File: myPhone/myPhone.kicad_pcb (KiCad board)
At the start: 2 copper layers, 135 x 70 mm, 211 parts, among them J1 USB_OTG, J2 BATT, J201 ESP32.UART, J202 Modem, J203 SIM_Card, J204 Motor, J205 Micro_SD_Card, J206 Camera, J207 GPS, J3 RV.Debug, J301 iMX8, J4 SJ-3571N, J5 Display, J6 Touch, Q1 MMBT3906, SW1 RESET, SW2 WAKE, SW201 BOOT, U1 BQ25895, U10 74HC595, U11 ICS-43434, U12 MAX98357A, U13 FT813Q, U14 FAN5333BSX, U2 TPS62293, U201 ESP32-WROOM, U202 SN74CBTLV3125, U203 TXB0104RGY, U204 TXB0104RGY, U205 DRV2605L, U206 SN74CBTLV3126, U207 TPS22917, U208 SN74LVC2G66, U209 TPS22917, U3 TPS630250, U4 SN74LVC2G07, U5 E310-G000, U6 IS25LP128-JBLE, U7 74HC00, U8 74HC00, U9 74HC595, X1 SiT1533, Y1 16MHz, Y2 12MHz

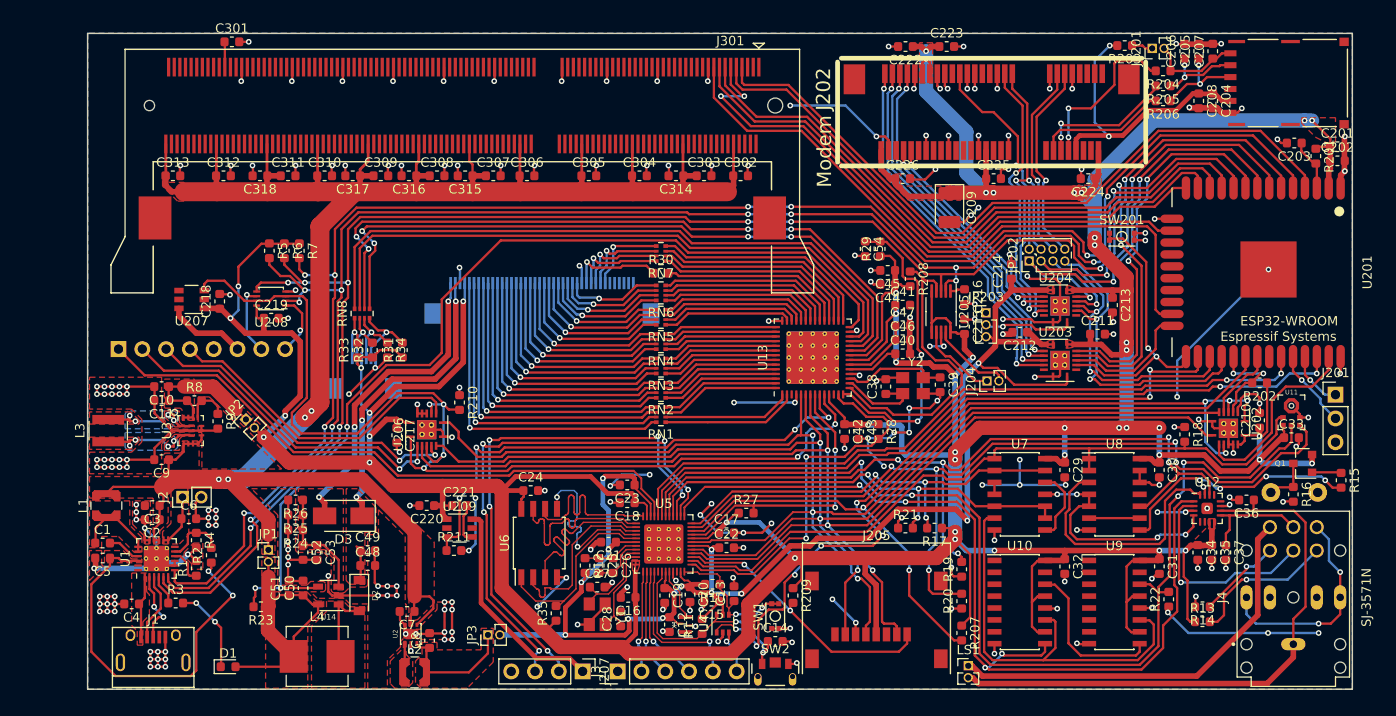
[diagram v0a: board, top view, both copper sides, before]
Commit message: REV1 board
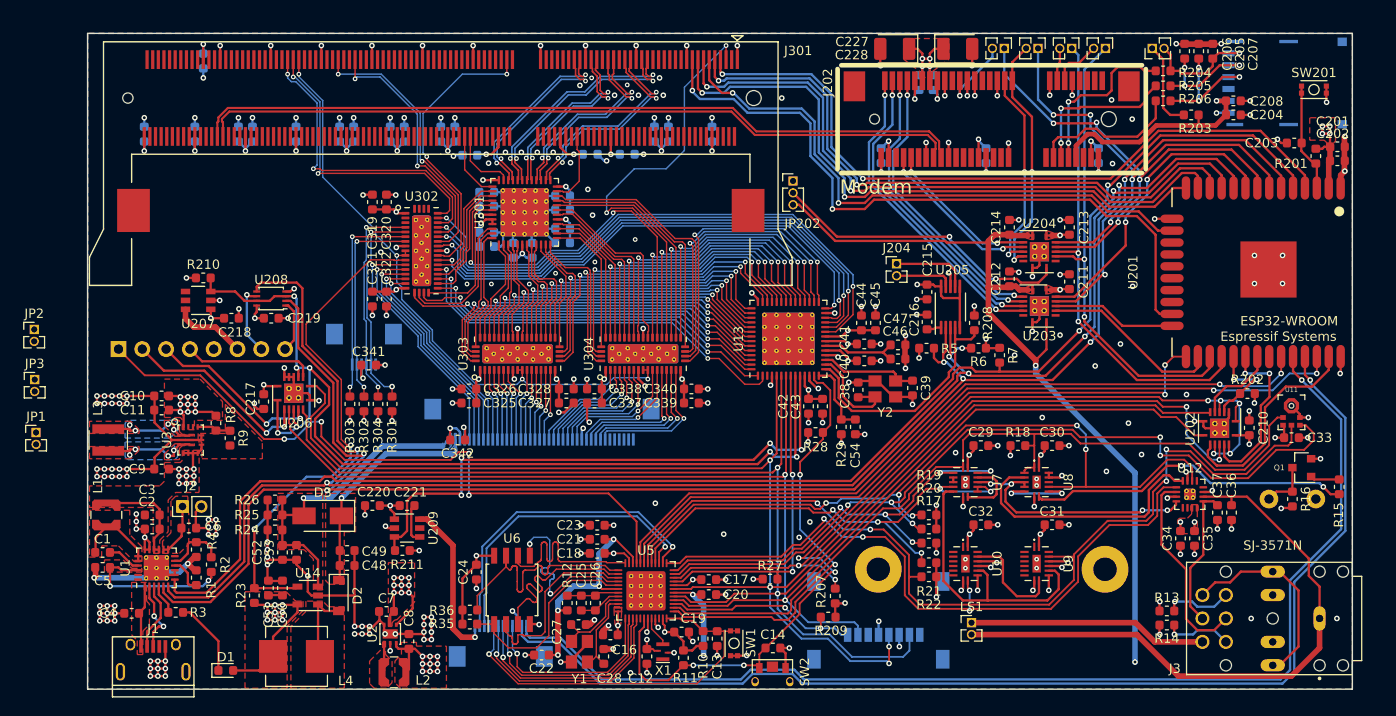
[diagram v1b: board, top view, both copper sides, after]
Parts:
- removed C15: 0.1uF, Capacitor_SMD:C_0603_1608Metric
- removed C209: 470uF, Capacitor_Tantalum_SMD:CP_EIA-3528-21_Kemet-B
- removed J201: ESP32.UART, Connector_PinHeader_2.54mm:PinHeader_1x03_P2.54mm_Vertical
- removed J207: GPS, Connector_PinHeader_2.54mm:PinHeader_1x04_P2.54mm_Vertical
- removed J4: SJ-3571N, footprints:CUI_SJ-3571N
- removed J5: Display, footprints:Hirose_FH12-40S-0.5SH_1x40-1MP_P0.50mm_Horizontal_Bottom
- removed J6: Touch, footprints:Hirose_FH12-6S-0.5SH_1x06-1MP_P0.50mm_Horizontal_Bottom
- removed the JP202 at (197.7, 96.1)
- removed R30: 33R, Resistor_SMD:R_0603_1608Metric
- removed RN1, RN2, RN3, RN4, RN5, RN6, RN7, RN8: 33R, footprints:R_Array_Convex_4x0402
- removed U4: SN74LVC2G07, Package_TO_SOT_SMD:SOT-363_SC-70-6
- added C227: 470uF, Capacitor_Tantalum_SMD:CP_EIA-3528-21_Kemet-B, F.Cu at (190.1, 73.5)
- added C228: 470uF, Capacitor_Tantalum_SMD:CP_EIA-3528-21_Kemet-B, F.Cu at (183.3, 73.5)
- added C319: 1uF, Capacitor_SMD:C_0603_1608Metric, F.Cu at (127.6, 89.8)
- added C320: 0.1uF, Capacitor_SMD:C_0603_1608Metric, F.Cu at (129.1, 89.8)
- added C321: 1uF, Capacitor_SMD:C_0603_1608Metric, F.Cu at (127.6, 100.2)
- added C322: 0.1uF, Capacitor_SMD:C_0603_1608Metric, F.Cu at (129.1, 100.2)
- added C323: 0.1uF, Capacitor_SMD:C_0603_1608Metric, B.Cu at (147.9, 90.7)
- added C324: 0.01uF, Capacitor_SMD:C_0603_1608Metric, B.Cu at (147.9, 89.2)
- added C325: 1uF, Capacitor_SMD:C_0603_1608Metric, F.Cu at (137.9, 111.2)
- added C326: 0.1uF, Capacitor_SMD:C_0603_1608Metric, F.Cu at (137.9, 109.8)
- added C327: 1uF, Capacitor_SMD:C_0603_1608Metric, F.Cu at (148.3, 111.2)
- added C328: 0.1uF, Capacitor_SMD:C_0603_1608Metric, F.Cu at (148.3, 109.8)
- added C329: 0.1uF, Capacitor_SMD:C_0603_1608Metric, B.Cu at (139.8, 94.5)
- added C330: 0.01uF, Capacitor_SMD:C_0603_1608Metric, B.Cu at (139.8, 93.0)
- added C331: 0.1uF, Capacitor_SMD:C_0603_1608Metric, B.Cu at (142.7, 95.0)
- added C332: 0.01uF, Capacitor_SMD:C_0603_1608Metric, B.Cu at (144.7, 95.0)
- added C333: 0.1uF, Capacitor_SMD:C_0603_1608Metric, B.Cu at (147.9, 94.2)
- added C334: 0.01uF, Capacitor_SMD:C_0603_1608Metric, B.Cu at (147.9, 92.7)
- added C335: 0.1uF, Capacitor_SMD:C_0603_1608Metric, B.Cu at (139.8, 88.8)
- added C336: 0.01uF, Capacitor_SMD:C_0603_1608Metric, B.Cu at (139.8, 90.2)
- added C337: 1uF, Capacitor_SMD:C_0603_1608Metric, F.Cu at (151.3, 111.2)
- added C338: 0.1uF, Capacitor_SMD:C_0603_1608Metric, F.Cu at (151.3, 109.8)
- added C339: 1uF, Capacitor_SMD:C_0603_1608Metric, F.Cu at (161.7, 111.2)
- added C340: 0.1uF, Capacitor_SMD:C_0603_1608Metric, F.Cu at (161.7, 109.8)
- added C341: 0.1uF, Capacitor_SMD:C_0603_1608Metric, F.Cu at (127.2, 107.2)
- added C342: 0.1uF, Capacitor_SMD:C_0603_1608Metric, F.Cu at (136.7, 115.2)
- added J302: Touch, Connector_FFC-FPC:Hirose_FH12-6S-0.5SH_1x06-1MP_P0.50mm_Horizontal, B.Cu at (126.7, 105.3)
- added J303: Display, Connector_FFC-FPC:Hirose_FH12-40S-0.5SH_1x40-1MP_P0.50mm_Horizontal, B.Cu at (145.7, 113.3)
- added J304: Prog, Connector_FFC-FPC:Hirose_FH12-12S-0.5SH_1x12-1MP_P0.50mm_Horizontal, B.Cu at (141.3, 136.9)
- added JP203: Q.DTR, Connector_PinHeader_1.27mm:PinHeader_1x02_P1.27mm_Vertical, F.Cu at (195.1, 73.4)
- added JP204: Q.RI, Connector_PinHeader_1.27mm:PinHeader_1x02_P1.27mm_Vertical, F.Cu at (198.7, 73.4)
- added JP205: Q.TXD, Connector_PinHeader_1.27mm:PinHeader_1x02_P1.27mm_Vertical, F.Cu at (202.2, 73.4)
- added JP206: Q.RXD, Connector_PinHeader_1.27mm:PinHeader_1x02_P1.27mm_Vertical, F.Cu at (205.8, 73.4)
- added R36: 100K, Resistor_SMD:R_0603_1608Metric, F.Cu at (138.0, 133.3)
- added U301: SN65LVDS822_SWAP, Package_DFN_QFN:QFN-48-1EP_7x7mm_P0.5mm_EP5.15x5.15mm_ThermalVias, F.Cu at (143.8, 90.9)
- added U302: TS3DDR3812, footprints:Texas_R-PWQFN-N42, F.Cu at (132.8, 95.0)
- added U303: TS3DDR3812, footprints:Texas_R-PWQFN-N42, F.Cu at (143.1, 106.0)
- added U304: TS3DDR3812, footprints:Texas_R-PWQFN-N42, F.Cu at (156.5, 106.0)
- C222, C223, C224, C225, C226, C301, C302, C303, C304, C305, C306, C307, C308, C309, C310, C311, C312, C313, C314, C315, C316, C317, C318, J203, J205: moved to B.Cu
- J3: value RV.Debug -> SJ-3571N; footprint Connector_PinHeader_2.54mm:PinHeader_1x06_P2.54mm_Vertical -> footprints:CUI_SJ-3571N
- R208: value 47K -> 100K
- U10, U9: footprint Package_SO:SOIC-16_3.9x9.9mm_P1.27mm -> footprints:74HC595BQ115
- U12: footprint Package_DFN_QFN:TQFN-16-1EP_3x3mm_P0.5mm_EP1.23x1.23mm -> footprints:TQFN-16-1EP_3x3mm_P0.5mm_EP1.23x1.23mm_ThermalVias
- U5: value E310-G000 -> E310-G002
- U7, U8: footprint Package_SO:SOIC-14_3.9x8.7mm_P1.27mm -> footprints:74HC00BQ115
- moved R7 75.6 mm to (194.6, 106.2)
- moved R6 74.8 mm to (192.3, 105.4), turned to 180 degrees
- moved R5 70.9 mm to (186.8, 105.4), turned to 0 degrees
- moved J3 70.1 mm to (223.7, 134.2), turned to 180 degrees
- moved JP3 55.5 mm to (91.5, 108.8), turned to 0 degrees
- moved R210 30.4 mm to (109.5, 97.9), turned to 0 degrees
- moved JP1 27.8 mm to (91.7, 114.4)
- moved SW201 25.8 mm to (228.1, 77.8)
- moved R22 25.7 mm to (187.0, 129.8), turned to 180 degrees
- moved JP202 25.0 mm to (172.5, 87.5)
- moved JP2 24.6 mm to (91.5, 103.4), turned to 0 degrees
- moved R29 19.4 mm to (177.7, 113.8)
- moved C54 19.0 mm to (179.2, 113.8)
- moved R18 17.8 mm to (196.5, 115.8), turned to 0 degrees
- moved J204 15.8 mm to (183.6, 96.4), turned to 0 degrees
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- renumbered C20 to C19, C22 to C20, C23 to C21, C19 to C22, C21 to C23, JP203 to JP202, R31 to R301, R32 to R302, R33 to R303, R34 to R304
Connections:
- net /DISP_LED_A renamed DISP_LED_A
- net /DISP_LED_K renamed DISP_LED_K
- net Net-(C25-Pad2) renamed /PLL_AVSS
- net Net-(C27-Pad1) renamed /XTAL_XI
- net Net-(C28-Pad1) renamed /XTAL_XO
- net Net-(R35-Pad2) renamed /QSPI_CS
- net Net-(U5-Pad1) renamed /QSPI_DQ_3
- net Net-(U5-Pad2) renamed /QSPI_DQ_2
- net Net-(U5-Pad20) renamed /PSD_LFALTCLK
- net Net-(U5-Pad3) renamed /QSPI_DQ_1
- net Net-(U5-Pad4) renamed /QSPI_DQ_0
- net Net-(U5-Pad48) renamed /QSPI_CLK
- C12 pad 1: +1V8 -> +3V3
- C13 pad 1: Net-(C13-Pad1) -> RESET
- C14 pad 1: Net-(C14-Pad1) -> WAKE
- C19 pad 1: +1V8 -> +3V3
- C23 pad 1: +1V8 -> +3V3
- C25 pad 1: Net-(C25-Pad1) -> /PLL_AVDD
- C26 pad 1: Net-(C25-Pad1) -> /PLL_AVDD
- J1 pad 4: (no net) -> Net-(J1-Pad4)
- J202 pad 1: (no net) -> Net-(J202-Pad1)
- J202 pad 16: (no net) -> Net-(J202-Pad16)
- J202 pad 20: (no net) -> Net-(J202-Pad20)
- J202 pad 22: (no net) -> Net-(J202-Pad22)
- J202 pad 23: (no net) -> Net-(J202-Pad23)
- J202 pad 25: (no net) -> Net-(J202-Pad25)
- J202 pad 28: (no net) -> Net-(J202-Pad28)
- J202 pad 3: (no net) -> Net-(J202-Pad3)
- J202 pad 30: (no net) -> Net-(J202-Pad30)
- J202 pad 32: (no net) -> Net-(J202-Pad32)
- J202 pad 33: (no net) -> Net-(J202-Pad33)
- J202 pad 36: (no net) -> iMX8_USB1_D_N
- J202 pad 38: (no net) -> iMX8_USB1_D_P
- J202 pad 42: (no net) -> Net-(J202-Pad42)
- J202 pad 48: (no net) -> Net-(J202-Pad48)
- J202 pad 5: (no net) -> Net-(J202-Pad5)
- J202 pad 6: (no net) -> Net-(J202-Pad6)
- J202 pad 7: (no net) -> Net-(J202-Pad7)
- J203 pad 6: (no net) -> Net-(J203-Pad6)
- J205 pad 3: (no net) -> Net-(J205-Pad3)
- J205 pad 8: (no net) -> Net-(J205-Pad8)
- J3 pad 1: GND -> /SPK_VO-
- J3 pad 2: JTAG_TCK -> Net-(J3-Pad2)
- J3 pad 3: JTAG_TDO -> Net-(J3-Pad2)
- J3 pad 4: JTAG_TMS -> Net-(J3-Pad4)
- J3 pad 5: JTAG_TDI -> /SPK_GAIN
- J3 pad 6: RESET -> Net-(J3-Pad6)
- J301 pad 100: (no net) -> Net-(J301-Pad100)
- J301 pad 101: (no net) -> Net-(J301-Pad101)
- J301 pad 102: (no net) -> Net-(J301-Pad102)
- J301 pad 103: (no net) -> Net-(J301-Pad103)
- J301 pad 104: (no net) -> Net-(J301-Pad104)
- J301 pad 106: (no net) -> Net-(J301-Pad106)
- J301 pad 107: (no net) -> Net-(J301-Pad107)
- J301 pad 108: (no net) -> Net-(J301-Pad108)
- J301 pad 109: (no net) -> Net-(J301-Pad109)
- J301 pad 110: (no net) -> Net-(J301-Pad110)
- J301 pad 111: (no net) -> Net-(J301-Pad111)
- J301 pad 112: (no net) -> Net-(J301-Pad112)
- J301 pad 113: (no net) -> Net-(J301-Pad113)
- J301 pad 115: (no net) -> Net-(J301-Pad115)
- J301 pad 116: (no net) -> Net-(J301-Pad116)
- J301 pad 117: (no net) -> Net-(J301-Pad117)
- J301 pad 118: (no net) -> Net-(J301-Pad118)
- J301 pad 119: (no net) -> Net-(J301-Pad119)
- J301 pad 12: (no net) -> Net-(J301-Pad12)
- J301 pad 120: (no net) -> Net-(J301-Pad120)
- J301 pad 121: (no net) -> Net-(J301-Pad121)
- J301 pad 122: (no net) -> Net-(J301-Pad122)
- J301 pad 124: (no net) -> Net-(J301-Pad124)
- J301 pad 125: (no net) -> Net-(J301-Pad125)
- J301 pad 126: (no net) -> Net-(J301-Pad126)
- J301 pad 127: (no net) -> Net-(J301-Pad127)
- J301 pad 128: (no net) -> Net-(J301-Pad128)
- J301 pad 129: (no net) -> iMX8_I2C1_SCL
- J301 pad 130: (no net) -> Net-(J301-Pad130)
- J301 pad 131: (no net) -> Net-(J301-Pad131)
- J301 pad 133: (no net) -> Net-(J301-Pad133)
- J301 pad 134: (no net) -> Net-(J301-Pad134)
- J301 pad 135: (no net) -> iMX8_I2C1_SDA
- J301 pad 136: (no net) -> Net-(J301-Pad136)
- J301 pad 137: (no net) -> Net-(J301-Pad137)
- J301 pad 138: (no net) -> Net-(J301-Pad138)
- J301 pad 139: (no net) -> Net-(J301-Pad139)
- J301 pad 14: (no net) -> Net-(J301-Pad14)
- J301 pad 140: (no net) -> Net-(J301-Pad140)
- J301 pad 142: (no net) -> Net-(J301-Pad142)
- J301 pad 143: (no net) -> Net-(J301-Pad143)
- J301 pad 144: (no net) -> Net-(J301-Pad144)
- J301 pad 145: (no net) -> Net-(J301-Pad145)
- J301 pad 146: (no net) -> Net-(J301-Pad146)
- J301 pad 147: (no net) -> Net-(J301-Pad147)
- J301 pad 148: (no net) -> Net-(J301-Pad148)
- J301 pad 149: (no net) -> iMX8_GPIO3_IO13
- J301 pad 151: (no net) -> iMX8_GPIO3_IO12
- J301 pad 152: (no net) -> Net-(J301-Pad152)
- J301 pad 153: (no net) -> iMX8_GPIO3_IO11
- J301 pad 154: (no net) -> Net-(J301-Pad154)
- J301 pad 155: (no net) -> Net-(J301-Pad155)
- J301 pad 156: (no net) -> Net-(J301-Pad156)
- J301 pad 157: (no net) -> Net-(J301-Pad157)
- J301 pad 158: (no net) -> Net-(J301-Pad158)
- J301 pad 16: (no net) -> Net-(J301-Pad16)
- J301 pad 160: (no net) -> Net-(J301-Pad160)
- J301 pad 161: (no net) -> Net-(J301-Pad161)
- J301 pad 162: (no net) -> Net-(J301-Pad162)
- J301 pad 163: (no net) -> Net-(J301-Pad163)
- J301 pad 164: (no net) -> Net-(J301-Pad164)
- J301 pad 165: (no net) -> Net-(J301-Pad165)
- J301 pad 166: (no net) -> Net-(J301-Pad166)
- J301 pad 167: (no net) -> Net-(J301-Pad167)
- J301 pad 169: (no net) -> Net-(J301-Pad169)
- J301 pad 170: (no net) -> Net-(J301-Pad170)
- J301 pad 171: (no net) -> Net-(J301-Pad171)
- J301 pad 172: (no net) -> Net-(J301-Pad172)
- J301 pad 173: (no net) -> Net-(J301-Pad173)
- J301 pad 174: (no net) -> Net-(J301-Pad174)
- J301 pad 175: (no net) -> Net-(J301-Pad175)
- J301 pad 176: (no net) -> iMX8_USB1_D_P
- J301 pad 178: (no net) -> iMX8_USB1_D_N
- J301 pad 179: (no net) -> Net-(J301-Pad179)
- J301 pad 18: (no net) -> Net-(J301-Pad18)
- J301 pad 180: (no net) -> Net-(J301-Pad180)
- J301 pad 181: (no net) -> Net-(J301-Pad181)
- J301 pad 182: (no net) -> Net-(J301-Pad182)
- J301 pad 184: (no net) -> Net-(J301-Pad184)
- J301 pad 185: (no net) -> Net-(J301-Pad185)
- J301 pad 187: (no net) -> Net-(J301-Pad187)
- J301 pad 188: (no net) -> Net-(J301-Pad188)
- J301 pad 189: (no net) -> Net-(J301-Pad189)
- J301 pad 190: (no net) -> Net-(J301-Pad190)
- J301 pad 191: (no net) -> Net-(J301-Pad191)
- J301 pad 192: (no net) -> Net-(J301-Pad192)
- J301 pad 193: (no net) -> Net-(J301-Pad193)
- J301 pad 194: (no net) -> Net-(J301-Pad194)
- J301 pad 195: (no net) -> Net-(J301-Pad195)
- J301 pad 196: (no net) -> Net-(J301-Pad196)
- J301 pad 197: (no net) -> Net-(J301-Pad197)
- J301 pad 198: (no net) -> Net-(J301-Pad198)
- J301 pad 199: (no net) -> Net-(J301-Pad199)
- J301 pad 2: (no net) -> Net-(J301-Pad2)
- J301 pad 20: (no net) -> Net-(J301-Pad20)
- J301 pad 200: (no net) -> Net-(J301-Pad200)
- J301 pad 201: (no net) -> Net-(J301-Pad201)
- J301 pad 202: (no net) -> Net-(J301-Pad202)
- J301 pad 203: (no net) -> Net-(J301-Pad203)
- J301 pad 21: (no net) -> Net-(J301-Pad21)
- J301 pad 22: (no net) -> Net-(J301-Pad22)
- J301 pad 23: (no net) -> Net-(J301-Pad23)
- J301 pad 24: (no net) -> Net-(J301-Pad24)
- J301 pad 25: (no net) -> Net-(J301-Pad25)
- J301 pad 26: (no net) -> Net-(J301-Pad26)
- J301 pad 27: (no net) -> Net-(J301-Pad27)
- J301 pad 29: (no net) -> Net-(J301-Pad29)
- J301 pad 3: (no net) -> Net-(J301-Pad3)
- J301 pad 30: (no net) -> Net-(J301-Pad30)
- J301 pad 31: (no net) -> Net-(J301-Pad31)
- J301 pad 32: (no net) -> Net-(J301-Pad32)
- J301 pad 33: (no net) -> iMX8_LVDS0_CLK_P
- J301 pad 34: (no net) -> Net-(J301-Pad34)
- J301 pad 35: (no net) -> iMX8_LVDS0_CLK_N
- J301 pad 36: (no net) -> Net-(J301-Pad36)
- J301 pad 38: (no net) -> Net-(J301-Pad38)
- J301 pad 39: (no net) -> iMX8_LVDS0_A0_P
- J301 pad 4: (no net) -> Net-(J301-Pad4)
- J301 pad 40: (no net) -> Net-(J301-Pad40)
- J301 pad 41: (no net) -> iMX8_LVDS0_A0_N
- J301 pad 42: (no net) -> Net-(J301-Pad42)
- J301 pad 43: (no net) -> Net-(J301-Pad43)
- J301 pad 44: (no net) -> Net-(J301-Pad44)
- J301 pad 45: (no net) -> iMX8_LVDS0_A1_P
- J301 pad 47: (no net) -> iMX8_LVDS0_A1_N
- J301 pad 48: (no net) -> Net-(J301-Pad48)
- J301 pad 49: (no net) -> Net-(J301-Pad49)
- J301 pad 5: (no net) -> iMX8_GPIO5_IO28
- J301 pad 50: (no net) -> Net-(J301-Pad50)
- J301 pad 51: (no net) -> iMX8_LVDS0_A2_P
- J301 pad 52: (no net) -> Net-(J301-Pad52)
- J301 pad 53: (no net) -> iMX8_LVDS0_A2_N
- J301 pad 54: (no net) -> Net-(J301-Pad54)
- J301 pad 56: (no net) -> Net-(J301-Pad56)
- J301 pad 57: (no net) -> iMX8_LVDS0_A3_P
- J301 pad 58: (no net) -> iMX8_GPIO5_IO25
- J301 pad 59: (no net) -> iMX8_LVDS0_A3_N
- J301 pad 6: (no net) -> Net-(J301-Pad6)
- J301 pad 60: (no net) -> Net-(J301-Pad60)
- J301 pad 61: (no net) -> Net-(J301-Pad61)
- J301 pad 62: (no net) -> Net-(J301-Pad62)
- J301 pad 63: (no net) -> Net-(J301-Pad63)
- J301 pad 65: (no net) -> Net-(J301-Pad65)
- J301 pad 66: (no net) -> Net-(J301-Pad66)
- J301 pad 67: (no net) -> Net-(J301-Pad67)
- J301 pad 68: (no net) -> Net-(J301-Pad68)
- J301 pad 69: (no net) -> Net-(J301-Pad69)
- J301 pad 70: (no net) -> Net-(J301-Pad70)
- J301 pad 72: (no net) -> Net-(J301-Pad72)
- J301 pad 73: (no net) -> Net-(J301-Pad73)
- J301 pad 74: (no net) -> Net-(J301-Pad74)
- J301 pad 75: (no net) -> iMX8_PWM1
- J301 pad 76: (no net) -> Net-(J301-Pad76)
- J301 pad 77: (no net) -> Net-(J301-Pad77)
- J301 pad 79: (no net) -> Net-(J301-Pad79)
- J301 pad 8: (no net) -> Net-(J301-Pad8)
- J301 pad 80: (no net) -> Net-(J301-Pad80)
- J301 pad 81: (no net) -> Net-(J301-Pad81)
- J301 pad 82: (no net) -> Net-(J301-Pad82)
- J301 pad 83: (no net) -> Net-(J301-Pad83)
- J301 pad 84: (no net) -> Net-(J301-Pad84)
- J301 pad 85: (no net) -> Net-(J301-Pad85)
- J301 pad 86: (no net) -> Net-(J301-Pad86)
- J301 pad 88: (no net) -> iMX8_GPIO2_IO17
- J301 pad 89: (no net) -> Net-(J301-Pad89)
- J301 pad 90: (no net) -> iMX8_GPIO2_IO18
- J301 pad 91: (no net) -> Net-(J301-Pad91)
- J301 pad 92: (no net) -> Net-(J301-Pad92)
- J301 pad 93: (no net) -> Net-(J301-Pad93)
- J301 pad 94: (no net) -> Net-(J301-Pad94)
- J301 pad 95: (no net) -> Net-(J301-Pad95)
- J301 pad 97: (no net) -> Net-(J301-Pad97)
- J301 pad 98: (no net) -> Net-(J301-Pad98)
- J301 pad 99: (no net) -> Net-(J301-Pad99)
- R10 pad 1: Net-(C13-Pad1) -> RESET
- R10 pad 2: +1V8 -> +3V3
- R11 pad 1: Net-(C14-Pad1) -> WAKE
- R11 pad 2: +1V8 -> +3V3
- R12 pad 1: Net-(C25-Pad1) -> +1V8
- R12 pad 2: +1V8 -> /PLL_AVDD
- R13 pad 2: Net-(J4-Pad6) -> Net-(J3-Pad6)
- R14 pad 1: Net-(J4-Pad4) -> Net-(J3-Pad4)
- R208 pad 1: FT813.GPIO3 -> GND
- R208 pad 2: +3V3 -> FT813.GPIO3
- R210 pad 2: FT813.GPIO1 -> FT813.GPIO0
- R211 pad 1: FT813.GPIO0 -> FT813.GPIO1
- R23 pad 2: /BL_PWM -> BL_PWM
- R301 pad 2: Net-(J6-Pad5) -> /exp/CTP_INT
- R302 pad 2: Net-(J6-Pad2) -> /exp/CTP_SDA
- R303 pad 2: Net-(J6-Pad1) -> /exp/CTP_SCL
- R304 pad 1: Net-(J6-Pad4) -> /exp/CTP_RST
- SW1 pad 2: Net-(C13-Pad1) -> RESET
- SW2 pad 1: Net-(C14-Pad1) -> WAKE
- SW201 pad 1: /periph/ESP32.PCM.SYNC -> Net-(C203-Pad1)
- U1 pad 12: (no net) -> Net-(U1-Pad12)
- U1 pad 23: (no net) -> Net-(U1-Pad23)
- U1 pad 24: (no net) -> Net-(U1-Pad24)
- U10 pad 1: (no net) -> Net-(U10-Pad1)
- U10 pad 15: (no net) -> Net-(U10-Pad15)
- U10 pad 2: (no net) -> Net-(U10-Pad2)
- U10 pad 3: (no net) -> Net-(U10-Pad3)
- U10 pad 4: (no net) -> Net-(U10-Pad4)
- U10 pad 5: (no net) -> Net-(U10-Pad5)
- U10 pad 6: (no net) -> Net-(U10-Pad6)
- U10 pad 7: (no net) -> Net-(U10-Pad7)
- U13 pad 1: Net-(RN1-Pad2) -> FT813_R1
- U13 pad 12: (no net) -> Net-(U13-Pad12)
- U13 pad 2: Net-(RN1-Pad1) -> FT813_R0
- U13 pad 23: /CTP_RST -> FT813_CTP_RST
- U13 pad 24: /CTP_INT -> FT813_CTP_INT
- U13 pad 25: /CTP_SCL -> FT813_CTP_SCL
- U13 pad 26: /CTP_SDA -> FT813_CTP_SDA
- U13 pad 28: /BL_PWM -> FT813_BL_PWM
- U13 pad 29: Net-(RN7-Pad4) -> FT813_DE
- U13 pad 3: (no net) -> Net-(U13-Pad3)
- U13 pad 30: Net-(RN7-Pad3) -> FT813_VSYNC
- U13 pad 31: Net-(RN7-Pad2) -> FT813_HSYNC
- U13 pad 32: Net-(RN7-Pad1) -> FT813_DISP
- U13 pad 33: Net-(R30-Pad2) -> FT813_PCLK
- U13 pad 34: Net-(RN6-Pad4) -> FT813_B7
- U13 pad 35: Net-(RN6-Pad3) -> FT813_B6
- U13 pad 36: Net-(RN6-Pad2) -> FT813_B5
- U13 pad 37: Net-(RN6-Pad1) -> FT813_B4
- U13 pad 38: Net-(RN5-Pad4) -> FT813_B3
- U13 pad 39: Net-(RN5-Pad3) -> FT813_B2
- U13 pad 40: Net-(RN5-Pad2) -> FT813_B1
- U13 pad 41: Net-(RN5-Pad1) -> FT813_B0
- U13 pad 43: Net-(RN4-Pad4) -> FT813_G7
- U13 pad 44: Net-(RN4-Pad3) -> FT813_G6
- U13 pad 45: Net-(RN4-Pad2) -> FT813_G5
- U13 pad 46: Net-(RN4-Pad1) -> FT813_G4
- U13 pad 47: Net-(RN3-Pad4) -> FT813_G3
- U13 pad 48: Net-(RN3-Pad3) -> FT813_G2
- U13 pad 49: Net-(RN3-Pad2) -> FT813_G1
- U13 pad 50: Net-(RN3-Pad1) -> FT813_G0
- U13 pad 51: Net-(RN2-Pad4) -> FT813_R7
- U13 pad 52: Net-(RN2-Pad3) -> FT813_R6
- U13 pad 53: Net-(RN2-Pad2) -> FT813_R5
- U13 pad 54: Net-(RN2-Pad1) -> FT813_R4
- U13 pad 55: Net-(RN1-Pad4) -> FT813_R3
- U13 pad 56: Net-(RN1-Pad3) -> FT813_R2
- U14 pad 4: /BL_PWM -> BL_PWM
- U201 pad 10: ESP32.I2C0.SDA -> ESP32.I2C0.SCL
- U201 pad 11: ESP32.I2C0.SCL -> ESP32.I2C0.SDA
- U201 pad 17: (no net) -> Net-(U201-Pad17)
- U201 pad 18: (no net) -> Net-(U201-Pad18)
- U201 pad 19: (no net) -> Net-(U201-Pad19)
- U201 pad 20: (no net) -> Net-(U201-Pad20)
- U201 pad 21: (no net) -> Net-(U201-Pad21)
- U201 pad 22: (no net) -> Net-(U201-Pad22)
- U201 pad 25: /periph/ESP32.PCM.SYNC -> WAKE
- U201 pad 26: WAKE -> /periph/ESP32.PCM.SYNC
- U201 pad 27: /periph/ESP32.U2.RXD -> /periph/ESP32.U2.TXD
- U201 pad 28: /periph/ESP32.U2.TXD -> /periph/ESP32.U2.RXD
- U201 pad 30: SPI1.SCK -> /periph/ESP32.VSPI.SCK
- U201 pad 32: (no net) -> Net-(U201-Pad32)
- U201 pad 34: Net-(J201-Pad2) -> ESP32.RXD0
- U201 pad 35: Net-(J201-Pad1) -> ESP32.TXD0
- U202 pad 11: GND -> SPI1.SCK
- U202 pad 12: GND -> /periph/ESP32.VSPI.SCK
- U202 pad 13: +3V3 -> SPI1.SS3
- U203 pad 6: (no net) -> Net-(U203-Pad6)
- U203 pad 9: (no net) -> Net-(U203-Pad9)
- U204 pad 12: /periph/ESP32.U2.RI -> /periph/ESP32.U2.DTR
- U204 pad 13: /periph/ESP32.U2.DTR -> /periph/ESP32.U2.RI
- U204 pad 2: /periph/SIMCom.UART.DTR -> /periph/SIMCom.UART.RI
- U204 pad 3: /periph/SIMCom.UART.RI -> /periph/SIMCom.UART.DTR
- U204 pad 6: (no net) -> Net-(U204-Pad6)
- U204 pad 9: (no net) -> Net-(U204-Pad9)
- U206 pad 1: FT813.GPIO1 -> FT813.GPIO0
- U206 pad 10: FT813.GPIO1 -> FT813.GPIO0
- U206 pad 4: FT813.GPIO1 -> FT813.GPIO0
- U207 pad 3: FT813.GPIO1 -> FT813.GPIO0
- U207 pad 4: (no net) -> Net-(U207-Pad4)
- U207 pad 5: (no net) -> Net-(U207-Pad5)
- U208 pad 3: FT813.GPIO1 -> FT813.GPIO0
- U208 pad 7: FT813.GPIO1 -> FT813.GPIO0
- U209 pad 3: FT813.GPIO0 -> FT813.GPIO1
- U209 pad 5: (no net) -> Net-(U209-Pad5)
- U209 pad 6: Net-(J207-Pad1) -> TPS.VOUT
- U5 pad 17: (no net) -> Net-(U5-Pad17)
- U5 pad 18: Net-(C14-Pad1) -> WAKE
- U5 pad 19: +1V8 -> +3V3
- U5 pad 22: (no net) -> Net-(U5-Pad22)
- U5 pad 23: +1V8 -> +3V3
- U5 pad 24: Net-(C13-Pad1) -> RESET
- U5 pad 7: Net-(C25-Pad1) -> /PLL_AVDD
- U8 pad 11: (no net) -> Net-(U8-Pad11)
- U9 pad 1: (no net) -> Net-(U9-Pad1)
- U9 pad 15: (no net) -> Net-(U9-Pad15)
- U9 pad 2: (no net) -> Net-(U9-Pad2)
- U9 pad 3: (no net) -> Net-(U9-Pad3)
- U9 pad 4: (no net) -> Net-(U9-Pad4)
- U9 pad 5: (no net) -> Net-(U9-Pad5)
- U9 pad 6: (no net) -> Net-(U9-Pad6)
- U9 pad 7: (no net) -> Net-(U9-Pad7)
- X1 pad 1: (no net) -> Net-(X1-Pad1)
- X1 pad 4: +1V8 -> +3V3
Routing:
- net +3V3: track 668.5 -> 217.7 mm, vias 45 -> 84
- net +VSYS: track 275.3 -> 111.1 mm, vias 4 -> 39
- net ESP32.TXD0: track 0.00 -> 124.7 mm, vias 0 -> 1
- net ESP32.RXD0: track 0.00 -> 123.5 mm, vias 0 -> 1
- net /BL_PWM: track 102.4 -> 0.00 mm, vias 3 -> 0
- net iMX8_USB1_D_N: track 0.00 -> 82.7 mm
- net iMX8_USB1_D_P: track 0.00 -> 81.5 mm
- net /CTP_RST: track 76.6 -> 0.00 mm, vias 4 -> 0
- net /CTP_INT: track 74.0 -> 0.00 mm, vias 4 -> 0
- net GND: track 489.1 -> 417.5 mm, vias 240 -> 285
- net /CTP_SCL: track 71.1 -> 0.00 mm
- net /CTP_SDA: track 68.6 -> 0.00 mm
- net iMX8_GPIO3_IO13: track 0.00 -> 66.1 mm, vias 0 -> 4
- net FT813_CTP_RST: track 0.00 -> 61.2 mm, vias 0 -> 2
- net FT813_CTP_INT: track 0.00 -> 59.3 mm, vias 0 -> 2
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- added copper zone on PWR, net +1V8
- added copper zone on PWR, net +3V3
- added copper zone on PWR, net +VSYS
- added copper zone on B.Cu, net DISP_LED_A
- added copper zone on B.Cu, net DISP_LED_K
- added copper zone on GND, net GND
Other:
- copper layers 2 -> 4
- net class DISPLAY added: clearance 0.1524, trace_width 0.1524, via_dia 0.508, via_drill 0.254
- net class Default: clearance 0.18 -> 0.2; via_dia 0.6096 -> 0.6; via_drill 0.3048 -> 0.3
- net class FE310_L added: clearance 0.2, trace_width 0.2, via_dia 0.6, via_drill 0.3
- net class MODEM_USB added: clearance 0.1524, trace_width 0.1524, via_dia 0.508, via_drill 0.254
- rule trace_clearance: 0.18 -> 0.2
- rule via_min_drill: 0.3 -> 0.2
